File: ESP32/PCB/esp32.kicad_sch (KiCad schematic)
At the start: 75 parts, among them J1 USB_C_Receptacle_USB2.0_14P, J2 Conn_01x02_Pin, J3 Conn_01x18_Pin, J5 Conn_01x18_Pin, Q1 AO3401A, U1 ESP32-S3, U2 W25Q128JVS, U3 MCP73831-2-OT, U4 AMS1117-3.3, Y1 32.768 kHz, Y2 40MHz(10ppm)

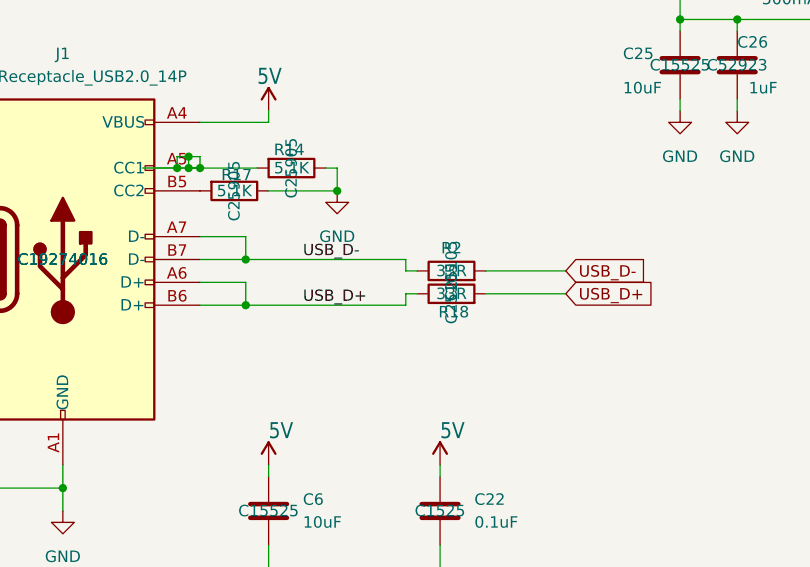
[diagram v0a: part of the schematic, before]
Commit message: Add files via upload
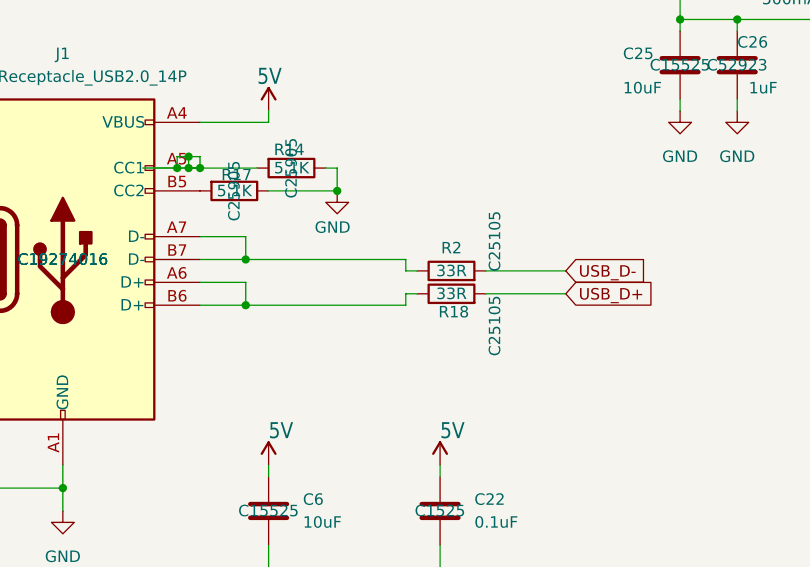
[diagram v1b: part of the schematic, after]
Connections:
- net USB_D+: no longer J1.A6 (D+), J1.B6 (D+), R18.1
- net USB_D-: no longer J1.A7 (D-), J1.B7 (D-), R2.1
- new net: J1.A6 (D+), J1.B6 (D+), R18.1
- new net: J1.A7 (D-), J1.B7 (D-), R2.1
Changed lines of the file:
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@@
 		)
 	)
-	(label "USB_D-"
-		(at 133.35 143.51 0)
-		(effects
-			(font
-				(size 1.2446 1.2446)
-			)
-			(justify left bottom)
-		)
-	)
-	(label "USB_D+"
-		(at 133.35 148.59 0)
-		(effects
-			(font
-				(size 1.2446 1.2446)
-			)
-			(justify left bottom)
-		)
-	)
 	(label "5V"
 		(at 347.98 176.53 0)
@@
 		)
 		(property "LCSC" "C25105"
-			(at 149.86 147.32 0)
+			(at 154.686 150.876 0)
 			(effects
 				(font
@@
 		)
 		(property "LCSC" "C25105"
-			(at 149.86 144.78 0)
+			(at 154.686 141.478 0)
 			(effects
 				(font
@@
 		)
 		(property "Value" "GND"
-			(at 137.16 140.97 0)
+			(at 136.652 139.954 0)
 			(effects
 				(font

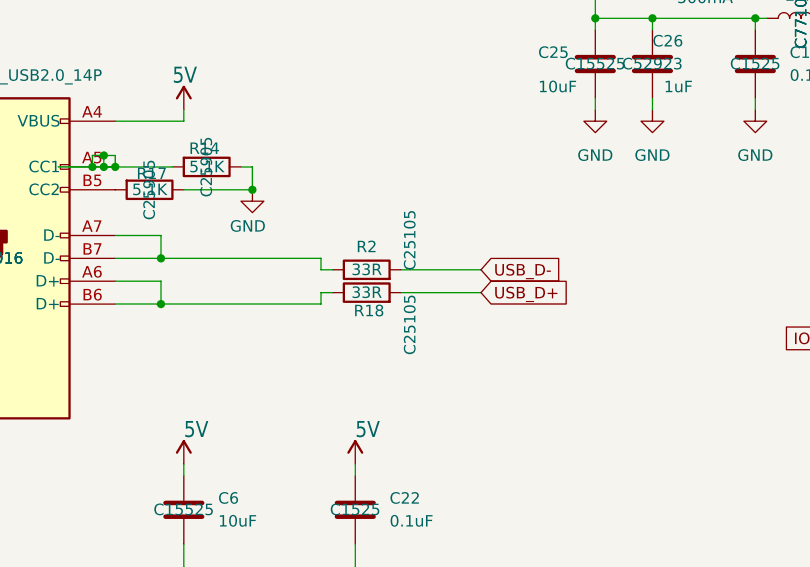
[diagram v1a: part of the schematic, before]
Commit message: Add files via upload
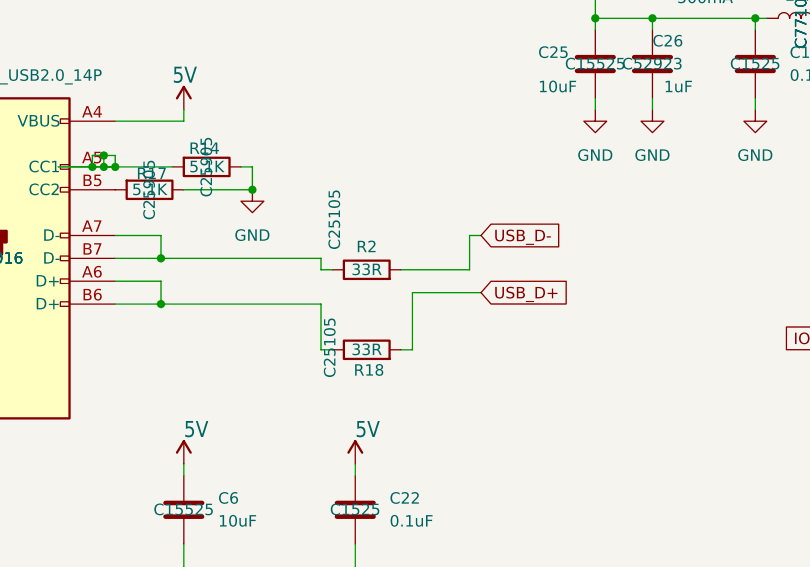
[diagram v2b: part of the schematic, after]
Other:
- moved on the sheet: R18
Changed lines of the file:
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@@
 	(wire
 		(pts
-			(xy 153.67 147.32) (xy 162.56 147.32)
+			(xy 153.67 153.67) (xy 154.94 153.67)
 		)
 		(stroke
@@
 	(wire
 		(pts
-			(xy 153.67 144.78) (xy 162.56 144.78)
+			(xy 161.29 140.97) (xy 162.56 140.97)
 		)
 		(stroke
@@
 	(wire
 		(pts
-			(xy 144.78 147.32) (xy 146.05 147.32)
+			(xy 144.78 153.67) (xy 146.05 153.67)
 		)
 		(stroke
@@
 	(wire
 		(pts
-			(xy 144.78 148.59) (xy 144.78 147.32)
+			(xy 144.78 153.67) (xy 144.78 148.59)
 		)
 		(stroke
@@
 	(wire
 		(pts
+			(xy 154.94 153.67) (xy 154.94 147.32)
+		)
+		(stroke
+			(width 0.1524)
+			(type solid)
+		)
+	)
+	(wire
+		(pts
 			(xy 210.82 147.32) (xy 205.74 147.32)
 		)
@@
 	(wire
 		(pts
+			(xy 154.94 147.32) (xy 162.56 147.32)
+		)
+		(stroke
+			(width 0.1524)
+			(type solid)
+		)
+	)
+	(wire
+		(pts
 			(xy 406.4 181.61) (xy 406.4 186.69)
 		)
@@
 	(wire
 		(pts
+			(xy 161.29 140.97) (xy 161.29 144.78)
+		)
+		(stroke
+			(width 0.1524)
+			(type solid)
+		)
+	)
+	(wire
+		(pts
 			(xy 177.8 215.9) (xy 172.72 215.9)
 		)
@@
 	(wire
 		(pts
+			(xy 161.29 144.78) (xy 153.67 144.78)
+		)
+		(stroke
+			(width 0.1524)
+			(type solid)
+		)
+	)
+	(wire
+		(pts
 			(xy 260.35 214.63) (xy 260.35 219.71)
 		)
@@
 	(global_label "USB_D-"
 		(shape input)
-		(at 162.56 144.78 0)
+		(at 162.56 140.97 0)
 		(fields_autoplaced yes)
 		(effects
@@
 		)
 		(property "Intersheetrefs" "${INTERSHEET_REFS}"
-			(at 173.1652 144.78 0)
+			(at 173.1652 140.97 0)
 			(effects
 				(font
@@
 	(symbol
 		(lib_id "Device:R")
-		(at 149.86 147.32 90)
+		(at 149.86 153.67 90)
 		(unit 1)
 		(exclude_from_sim no)
@@
 		(dnp no)
 		(property "Reference" "R18"
-			(at 150.114 149.352 90)
+			(at 150.114 155.956 90)
 			(effects
 				(font
@@
 		)
 		(property "Value" "33R"
-			(at 149.86 147.32 90)
+			(at 149.86 153.67 90)
 			(effects
 				(font
@@
 		)
 		(property "Footprint" "Resistor_SMD:R_0402_1005Metric"
-			(at 149.86 149.098 90)
+			(at 149.86 155.448 90)
 			(effects
 				(font
@@
 		)
 		(property "Datasheet" "~"
-			(at 149.86 147.32 0)
+			(at 149.86 153.67 0)
 			(effects
 				(font
@@
 		)
 		(property "Description" ""
-			(at 149.86 147.32 0)
+			(at 149.86 153.67 0)
 			(effects
 				(font
@@
 		)
 		(property "MNF PART NUMBER" "C25105"
-			(at 149.86 147.32 0)
+			(at 149.86 153.67 0)
 			(effects
 				(font
@@
 		)
 		(property "Sim.Device" ""
-			(at 149.86 147.32 0)
+			(at 149.86 153.67 0)
 			(effects
 				(font
@@
 		)
 		(property "Sim.Pins" ""
-			(at 149.86 147.32 0)
+			(at 149.86 153.67 0)
 			(effects
 				(font
@@
 		)
 		(property "PARTNO" ""
-			(at 149.86 147.32 0)
+			(at 149.86 153.67 0)
 			(effects
 				(font
@@
 		)
 		(property "LCSC" "C25105"
-			(at 154.686 150.876 0)
+			(at 145.796 153.416 0)
 			(effects
 				(font
@@
 		)
 		(property "LCSC" "C25105"
-			(at 154.686 141.478 0)
+			(at 146.304 139.192 0)
 			(effects
 				(font
@@
 		)
 		(property "Value" "GND"
-			(at 136.652 139.954 0)
+			(at 137.16 140.97 0)
 			(effects
 				(font
